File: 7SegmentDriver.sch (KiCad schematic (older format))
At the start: 5 parts, among them U10 ULN2003, U6 CD4514, U7 CD4511, U8 ULN2003, U9 ULN2003

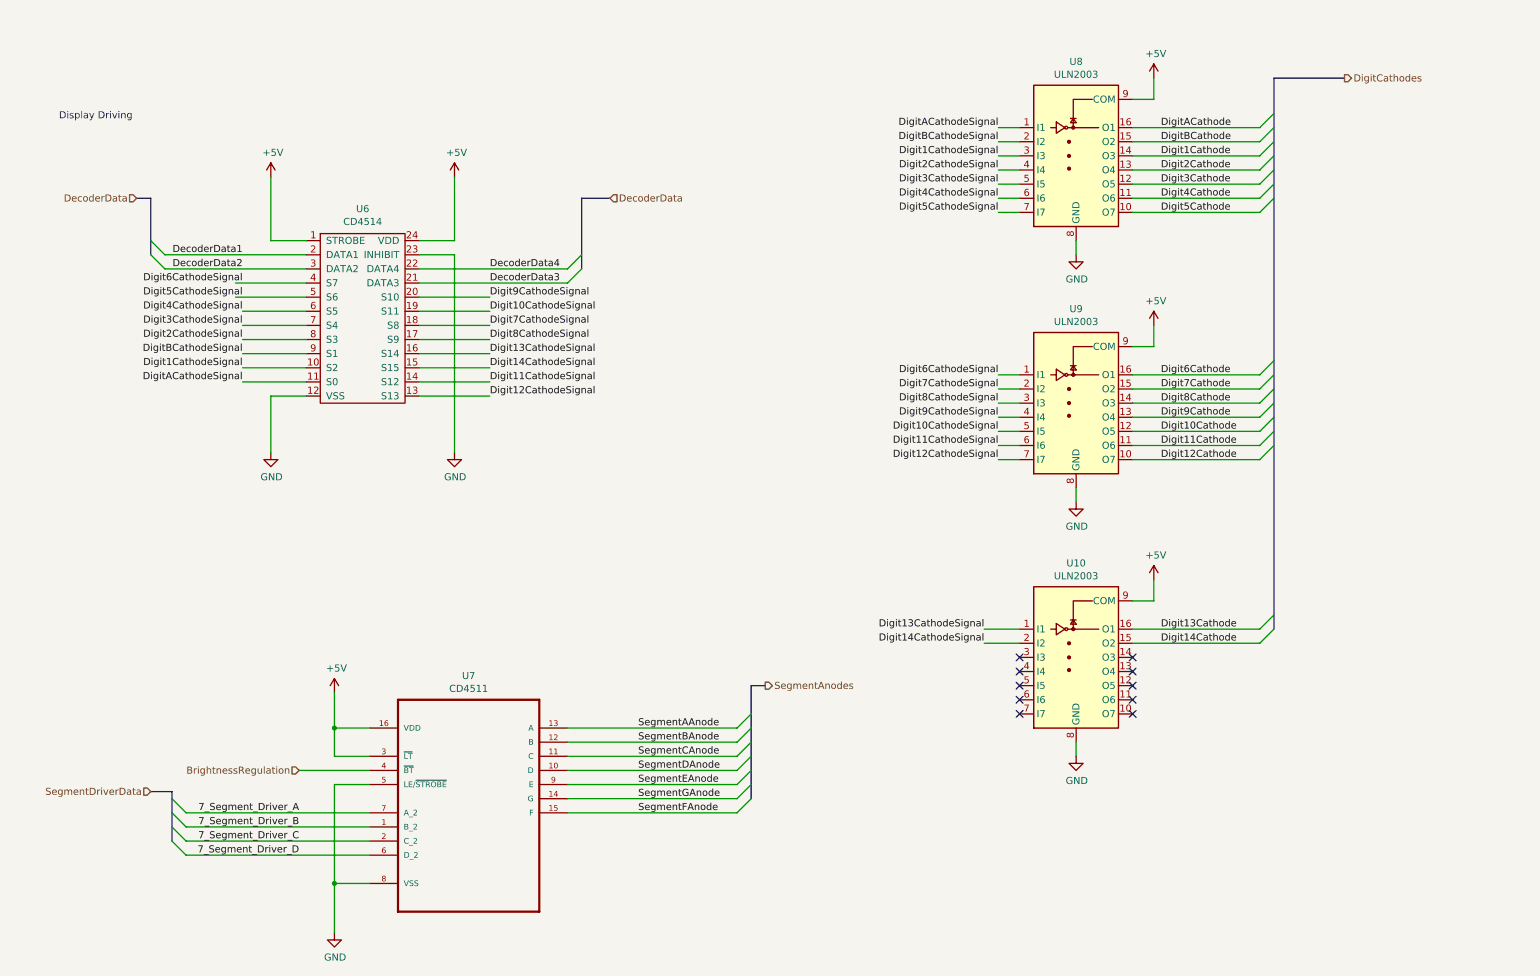
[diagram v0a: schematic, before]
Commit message: - Zwischenstand Display Driving
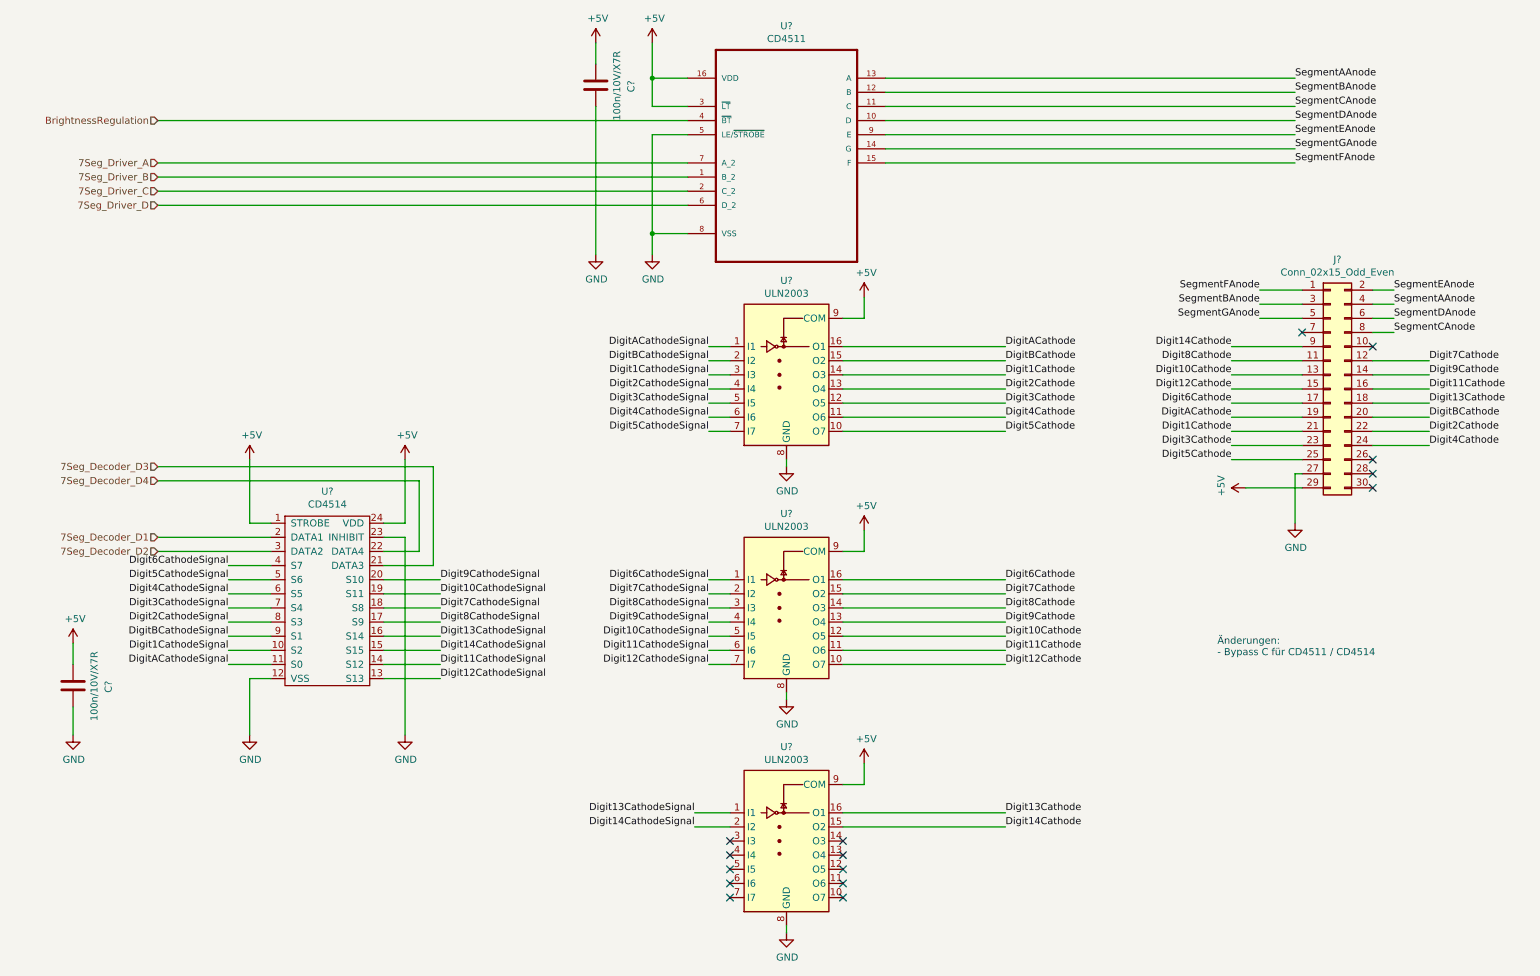
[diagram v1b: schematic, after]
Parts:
- removed U10, U8, U9: ULN2003, symbol Transistor_Array:ULN2003
- removed U6: CD4514, Package_SO:SOIC-24W_7.5x15.4mm_P1.27mm, symbol TeKaDe:CD4514
- removed U7: CD4511, Package_SO:SOIC-24W_7.5x15.4mm_P1.27mm, symbol TeKaDe:CD4511BE
- added C? (x2): 100n/10V/X7R, Resistor_SMD:R_0603_1608Metric, symbol Device:C
- added J?: Conn_02x15_Odd_Even, Connector_PinSocket_2.54mm:PinSocket_2x15_P2.54mm_Vertical, symbol Connector_Generic:Conn_02x15_Odd_Even
- added U? (x3): ULN2003, symbol Transistor_Array:ULN2003
- added U?: CD4511, Package_SO:SOIC-24W_7.5x15.4mm_P1.27mm, symbol TeKaDe:CD4511BE
- added U?: CD4514, Package_SO:SOIC-24W_7.5x15.4mm_P1.27mm, symbol TeKaDe:CD4514
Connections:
- net +5V: now also C?.1, C?.1, J?.29 (Pin_29), U?.1 (STROBE), U?.16 (VDD), U?.24 (VDD), U?.3 (~LT), U?.9 (COM), U?.9 (COM), U?.9 (COM)
- net BrightnessRegulation: now also U?.4 (~BT)
- net Digit10Cathode: now also J?.13 (Pin_13), U?.12 (O5)
- net Digit10CathodeSignal: now also U?.19 (S11), U?.5 (I5)
- net Digit11Cathode: now also J?.16 (Pin_16), U?.11 (O6)
- net Digit11CathodeSignal: now also U?.14 (S12), U?.6 (I6)
- net Digit12Cathode: now also J?.15 (Pin_15), U?.10 (O7)
- net Digit12CathodeSignal: now also U?.13 (S13), U?.7 (I7)
- net Digit13Cathode: now also J?.18 (Pin_18), U?.16 (O1)
- net Digit13CathodeSignal: now also U?.1 (I1), U?.16 (S14)
- net Digit14Cathode: now also J?.9 (Pin_9), U?.15 (O2)
- net Digit14CathodeSignal: now also U?.15 (S15), U?.2 (I2)
- net Digit1Cathode: now also J?.21 (Pin_21), U?.14 (O3)
- net Digit1CathodeSignal: now also U?.10 (S2), U?.3 (I3)
- net Digit2Cathode: now also J?.22 (Pin_22), U?.13 (O4)
- net Digit2CathodeSignal: now also U?.4 (I4), U?.8 (S3)
- net Digit3Cathode: now also J?.23 (Pin_23), U?.12 (O5)
- net Digit3CathodeSignal: now also U?.5 (I5), U?.7 (S4)
- net Digit4Cathode: now also J?.24 (Pin_24), U?.11 (O6)
- net Digit4CathodeSignal: now also U?.6 (I6), U?.6 (S5)
- net Digit5Cathode: now also J?.25 (Pin_25), U?.10 (O7)
- net Digit5CathodeSignal: now also U?.5 (S6), U?.7 (I7)
- net Digit6Cathode: now also J?.17 (Pin_17), U?.16 (O1)
- net Digit6CathodeSignal: now also U?.1 (I1), U?.4 (S7)
- net Digit7Cathode: now also J?.12 (Pin_12), U?.15 (O2)
- net Digit7CathodeSignal: now also U?.18 (S8), U?.2 (I2)
- net Digit8Cathode: now also J?.11 (Pin_11), U?.14 (O3)
- net Digit8CathodeSignal: now also U?.17 (S9), U?.3 (I3)
- net Digit9Cathode: now also J?.14 (Pin_14), U?.13 (O4)
- net Digit9CathodeSignal: now also U?.20 (S10), U?.4 (I4)
- net DigitACathode: now also J?.19 (Pin_19), U?.16 (O1)
- net DigitACathodeSignal: now also U?.1 (I1), U?.11 (S0)
- net DigitBCathode: now also J?.20 (Pin_20), U?.15 (O2)
- net DigitBCathodeSignal: now also U?.2 (I2), U?.9 (S1)
- net GND: now also C?.2, C?.2, J?.27 (Pin_27), U?.12 (VSS), U?.23 (INHIBIT), U?.5 (LE/~STROBE), U?.8 (GND), U?.8 (GND), U?.8 (GND), U?.8 (VSS)
- net SegmentAAnode: now also J?.4 (Pin_4), U?.13 (A)
- net SegmentBAnode: now also J?.3 (Pin_3), U?.12 (B)
- net SegmentCAnode: now also J?.8 (Pin_8), U?.11 (C)
- net SegmentDAnode: now also J?.6 (Pin_6), U?.10 (D)
- net SegmentEAnode: now also J?.2 (Pin_2), U?.9 (E)
- net SegmentFAnode: now also J?.1 (Pin_1), U?.15 (F)
- net SegmentGAnode: now also J?.5 (Pin_5), U?.14 (G)
- new net 7Seg_Decoder_D1: U?.2 (DATA1)
- new net 7Seg_Decoder_D2: U?.3 (DATA2)
- new net 7Seg_Decoder_D3: U?.21 (DATA3)
- new net 7Seg_Decoder_D4: U?.22 (DATA4)
- new net 7Seg_Driver_A: U?.7 (A_2)
- new net 7Seg_Driver_B: U?.1 (B_2)
- new net 7Seg_Driver_C: U?.2 (C_2)
- new net 7Seg_Driver_D: U?.6 (D_2)
- no-connect marks 10 -> 15
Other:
- note added: "Änderungen:\n- Bypass C für CD4511 / CD4514"
- note removed: "Display Driving"
